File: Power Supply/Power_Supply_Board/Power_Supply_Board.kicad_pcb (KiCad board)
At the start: 2 copper layers, 36 parts

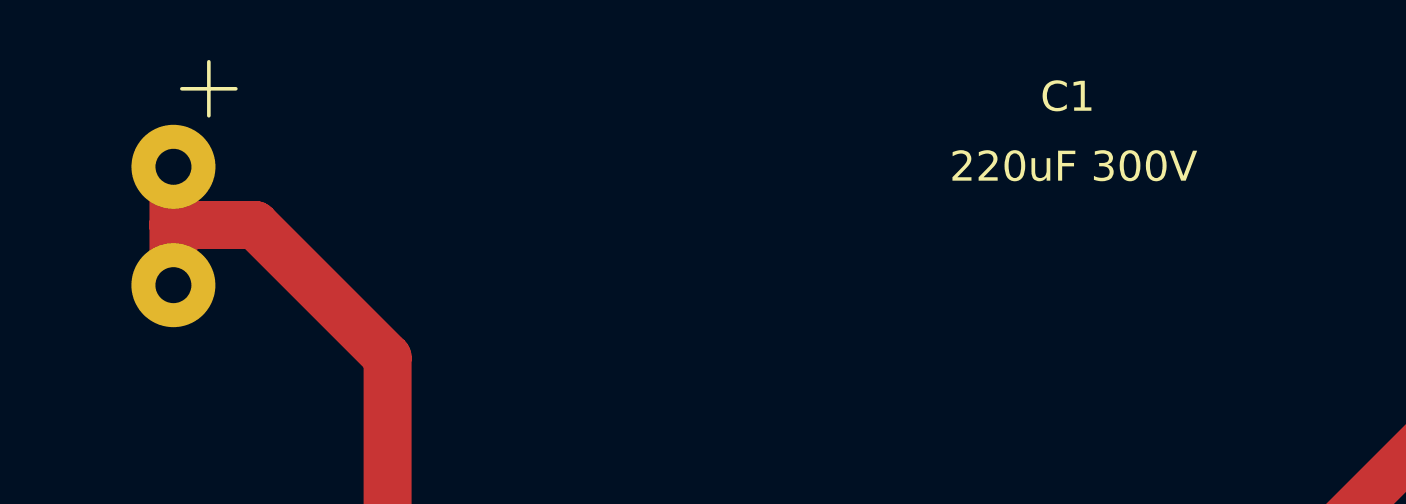
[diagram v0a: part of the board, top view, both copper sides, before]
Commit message: Power Supply Board Progress
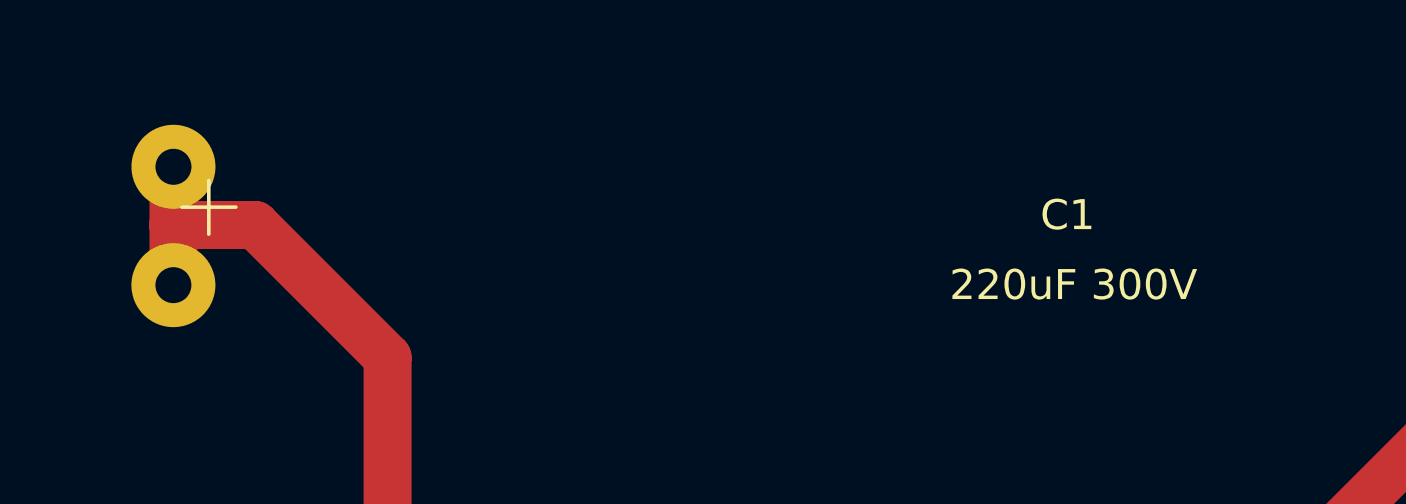
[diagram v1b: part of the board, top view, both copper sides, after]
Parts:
- moved C1 3.95 mm to (90.3, 86.7)
- moved C2 3.95 mm to (90.3, 82.7)
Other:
- board text removed: "Might not need the reservoir cap labels. just keep a little buffer on the edge, but otherwise, order doesnt matter just polarity"
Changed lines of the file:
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@@
 	(footprint "Capacitor_THT:CP_Axial_L55.0mm_D26.0mm_P60.00mm_Horizontal"
 		(layer "F.Cu")
-		(at 90.302 82.7075)
+		(at 90.3 86.6525)
 		(descr "CP, Axial series, Axial, Horizontal, pin pitch=60mm, , length*diameter=55*26mm^2, Electrolytic Capacitor, , http://www.vishay.com/docs/42037/53d.pdf")
 		(tags "CP Axial series Axial Horizontal pin pitch 60mm  length 55mm diameter 26mm Electrolytic Capacitor")
@@
 	(footprint "Capacitor_THT:CP_Axial_L55.0mm_D26.0mm_P60.00mm_Horizontal"
 		(layer "B.Cu")
-		(at 90.3 86.6525)
+		(at 90.302 82.7075)
 		(descr "CP, Axial series, Axial, Horizontal, pin pitch=60mm, , length*diameter=55*26mm^2, Electrolytic Capacitor, , http://www.vishay.com/docs/42037/53d.pdf")
 		(tags "CP Axial series Axial Horizontal pin pitch 60mm  length 55mm diameter 26mm Electrolytic Capacitor")
@@
 		)
 		(property "Value" "220uF 300V"
-			(at 30.43 -2.4 180)
+			(at 30.348 1.7475 180)
 			(layer "B.SilkS")
 			(effects
@@
 			)
 			(justify left bottom)
-		)
-	)
-	(gr_text "Might not need the reservoir cap labels. just keep a little buffer on the edge, but otherwise, order doesnt matter just polarity"
-		(at 94.2 72.26 0)
-		(layer "Edge.Cuts")
-		(effects
-			(font
-				(size 1 1)
-				(thickness 0.15)
-			)
-			(justify left bottom)
